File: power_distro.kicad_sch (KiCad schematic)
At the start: 33 parts, among them J1 Conn_01x02, J2 Conn_01x02, J3 Conn_01x02, J4 Conn_01x02, J5 Conn_01x02, J6 Conn_01x02, J7 Conn_01x02, J8 Conn_01x02

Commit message: schema change
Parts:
- J_IN1: footprint Connector_Phoenix_MSTB:PhoenixContact_MSTBVA_2,5_2-G-5,08_1x02_P5.08mm_Vertical -> TerminalBlock_MetzConnect:TerminalBlock_MetzConnect_Type171_RT13702HBWC_1x02_P7.50mm_Horizontal
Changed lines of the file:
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@@
 			)
 		)
-		(property "Footprint" "Connector_Phoenix_MSTB:PhoenixContact_MSTBVA_2,5_2-G-5,08_1x02_P5.08mm_Vertical"
+		(property "Footprint" "TerminalBlock_MetzConnect:TerminalBlock_MetzConnect_Type171_RT13702HBWC_1x02_P7.50mm_Horizontal"
 			(at 132.08 52.07 0)
 			(effects

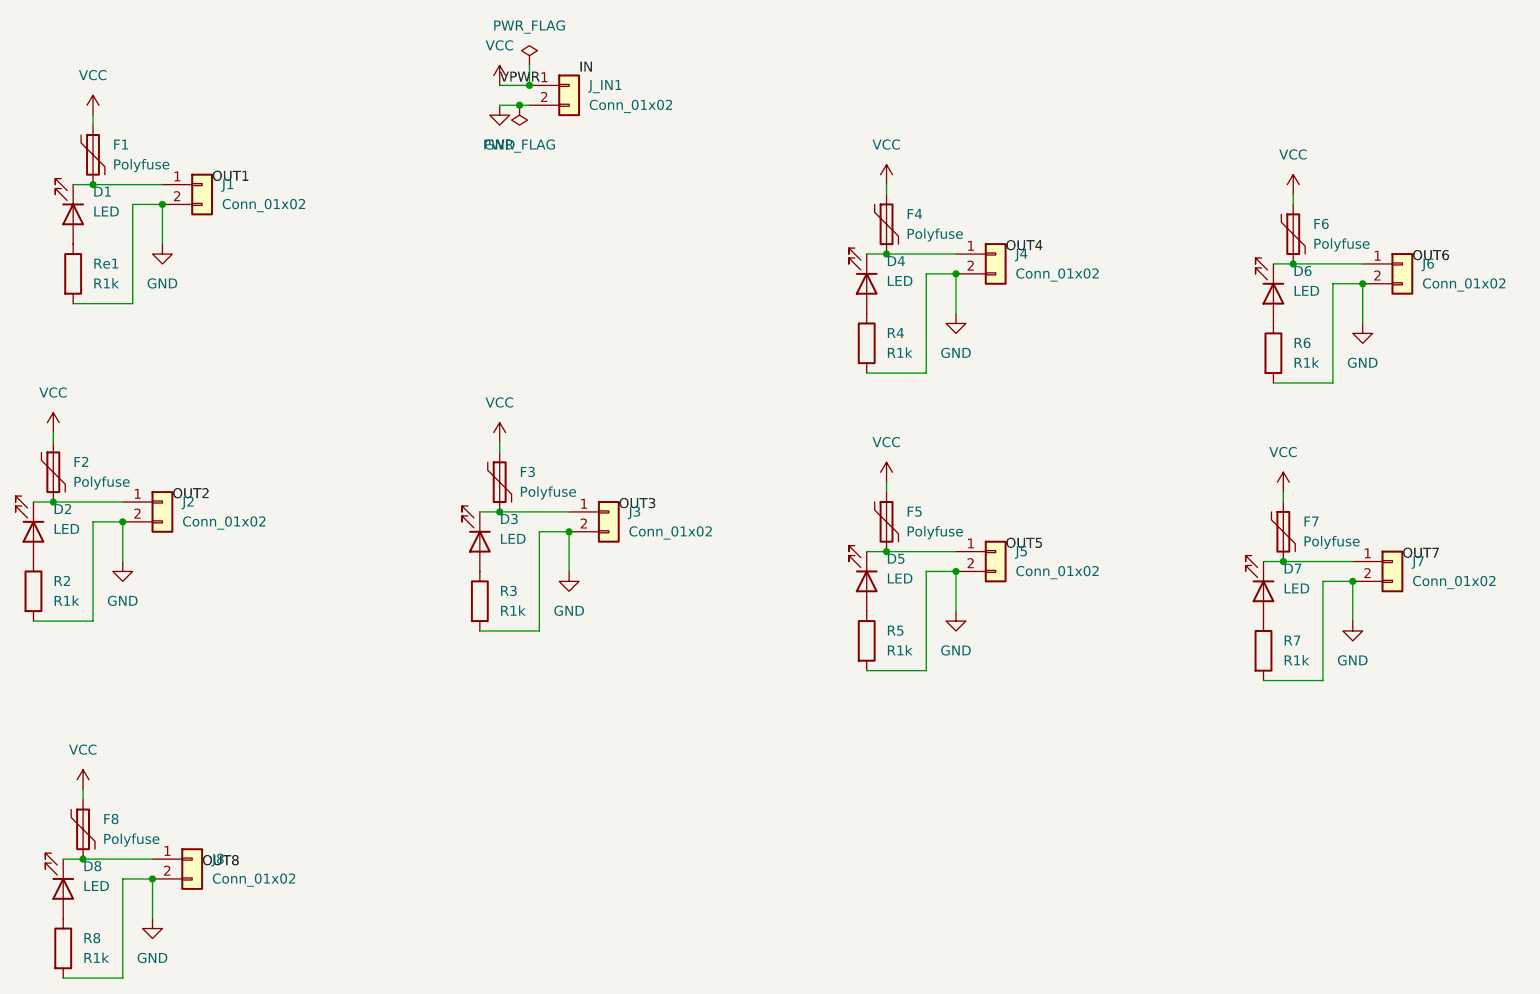
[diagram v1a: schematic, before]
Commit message: update for PTC
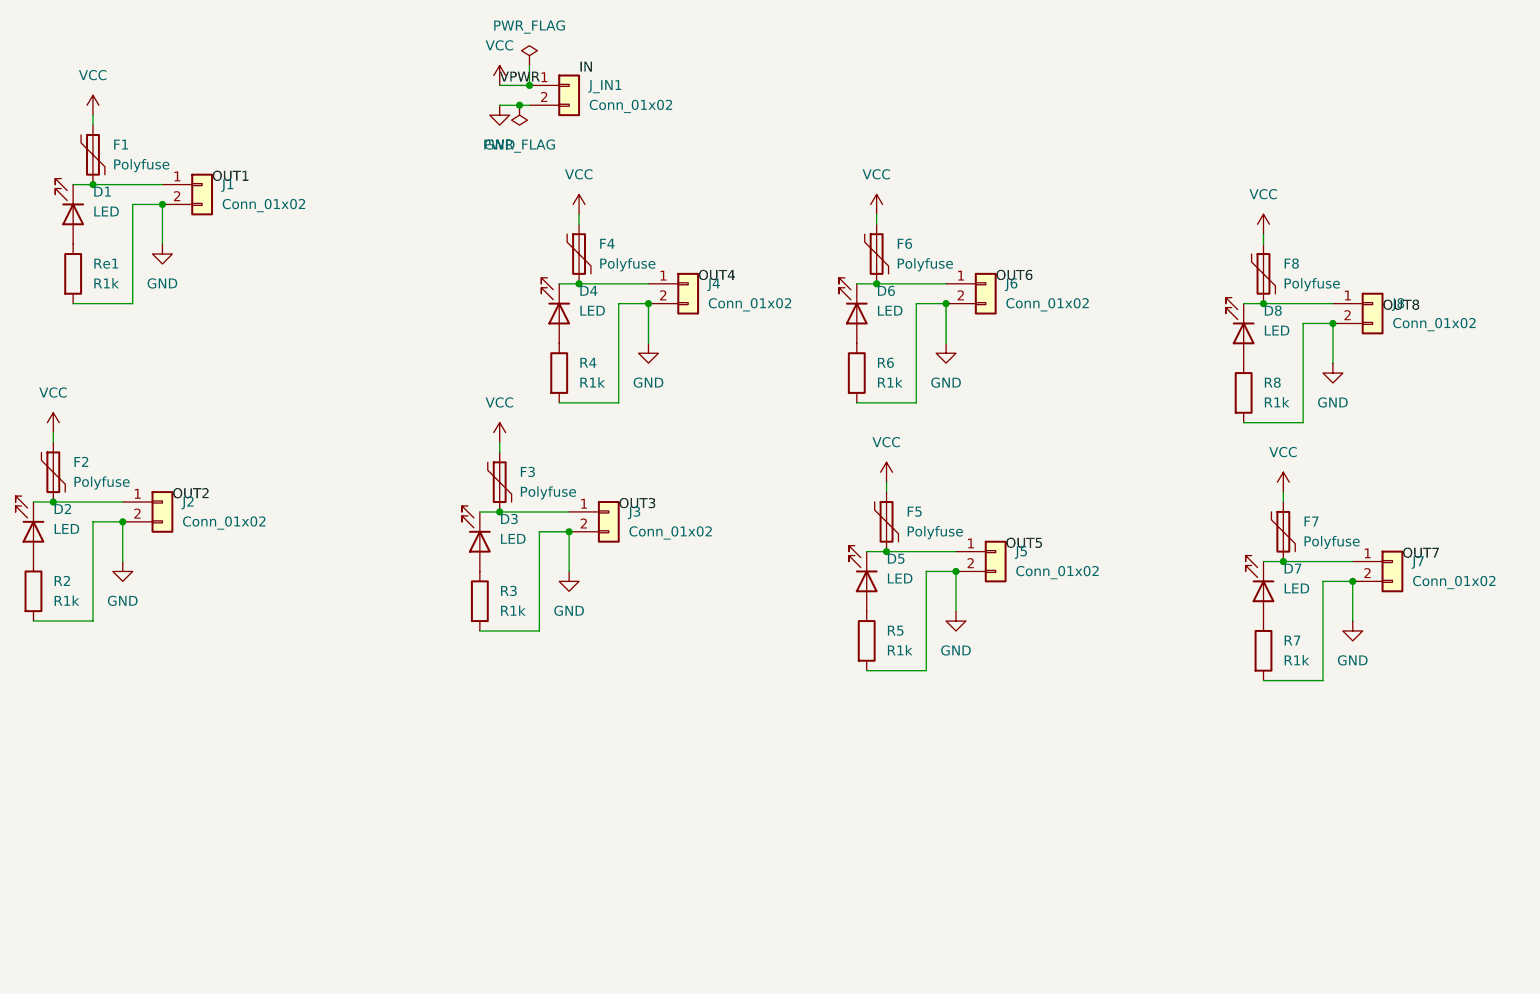
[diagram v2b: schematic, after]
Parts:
- F1, F2, F3, F4, F5, F6, F7, F8: footprint Fuse:Fuse_Bourns_MF-RHT500 -> Fuse:Fuse_Bourns_MF-RHT1000
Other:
- moved on the sheet: D4, D6, D8, F4, F6, F8, J4, J6, J8, R4, R6, R8
